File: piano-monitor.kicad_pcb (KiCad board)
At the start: 2 copper layers, 173.6 x 79 mm, 7 parts, among them J3 NCJ6FA-V, J4 DC, J5 230AC, J7 NCJ6FA-V

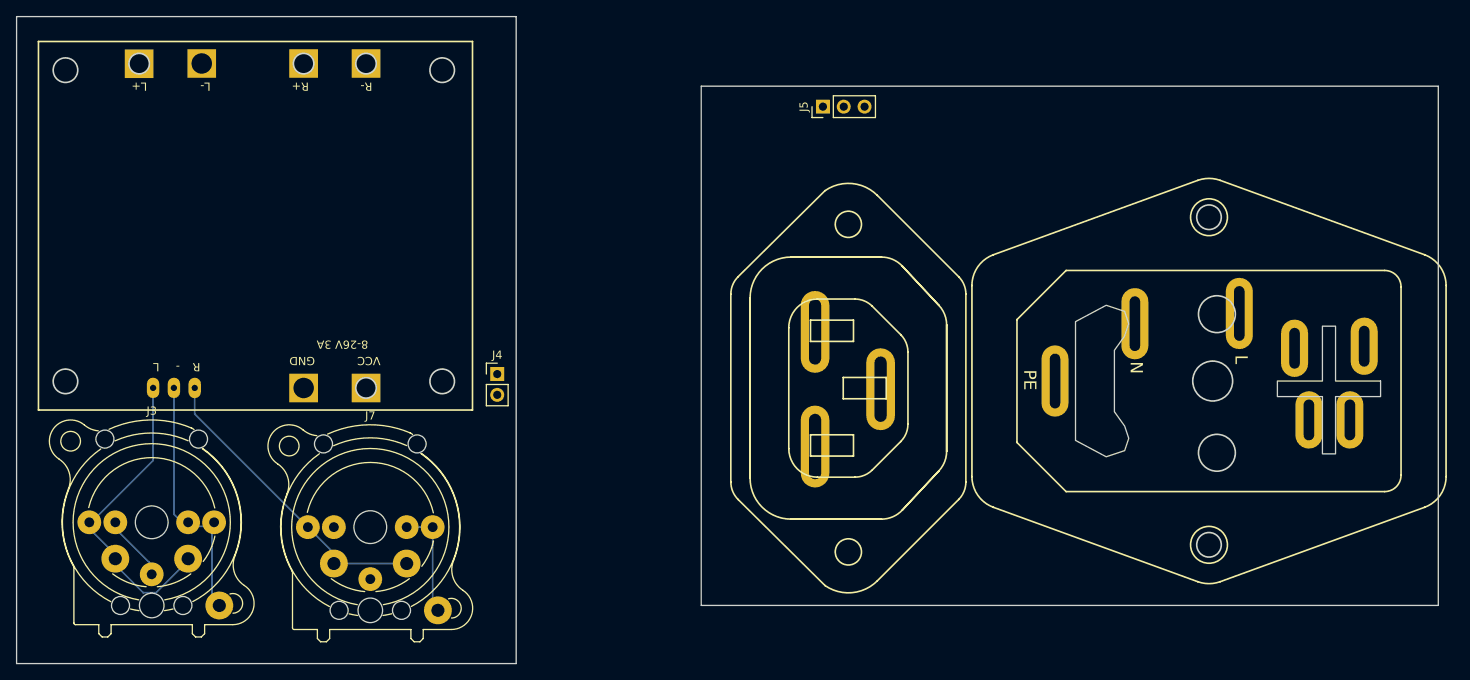
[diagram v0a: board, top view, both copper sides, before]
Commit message: Add some traces
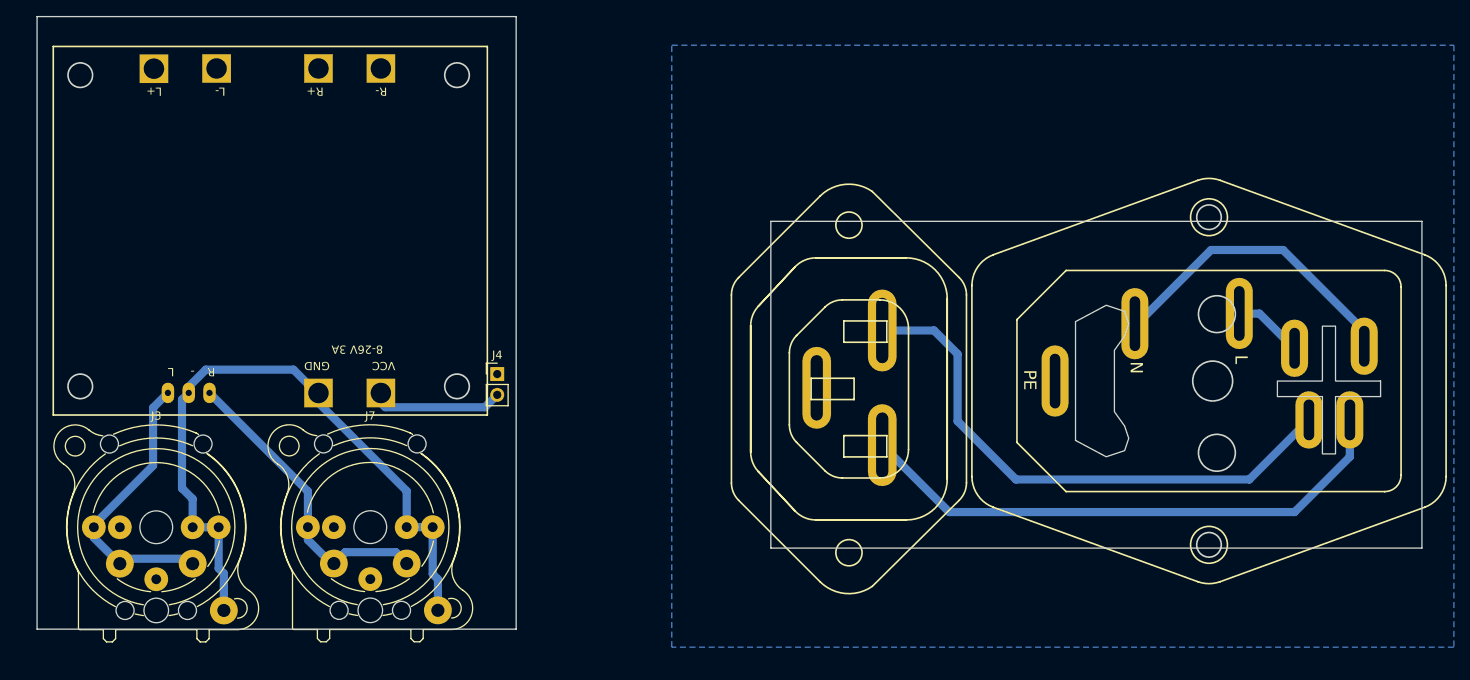
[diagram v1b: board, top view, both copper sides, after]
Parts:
- removed J5: 230AC, Connector_PinHeader_2.54mm:PinHeader_1x03_P2.54mm_Vertical
- moved U1 1.91 mm to (139.0, 77.8)
- moved J3 0.82 mm to (132.7, 113.9)
- turned J6 to -90 degrees
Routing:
- net L: track 0.00 -> 67.8 mm
- net N: track 0.00 -> 67.4 mm
- net S1: track 44.7 -> 84.0 mm
- net Net-(J1-B): track 0.00 -> 37.4 mm
- net +24V: track 0.00 -> 16.3 mm
- net R2: track 8.19 -> 0.00 mm
- net Net-(J1-A): track 0.00 -> 7.98 mm
- net T2: track 38.2 -> 35.6 mm
- added copper zone on B.Cu, net Earth
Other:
- board size 173.6 x 79 mm -> 169.1 x 74.8 mm
